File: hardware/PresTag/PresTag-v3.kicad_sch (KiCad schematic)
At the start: 20 parts, among them J201 CONN_02X04, J301 Conn_01x01, J302 Conn_01x01, J303 Conn_01x01, J304 Conn_01x01, J401 CONN_01X02, Q501 Q_NPN_BEC, U1 at25ex321D-UUN, U2 LPS27HHWTR, U302 stm32l412kb, U501 RV-3028-C7

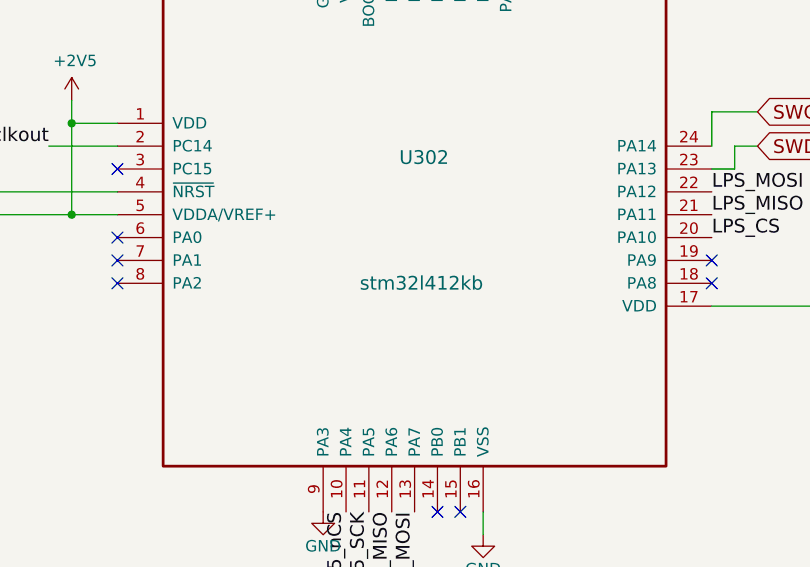
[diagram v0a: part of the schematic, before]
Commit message: revise prestag
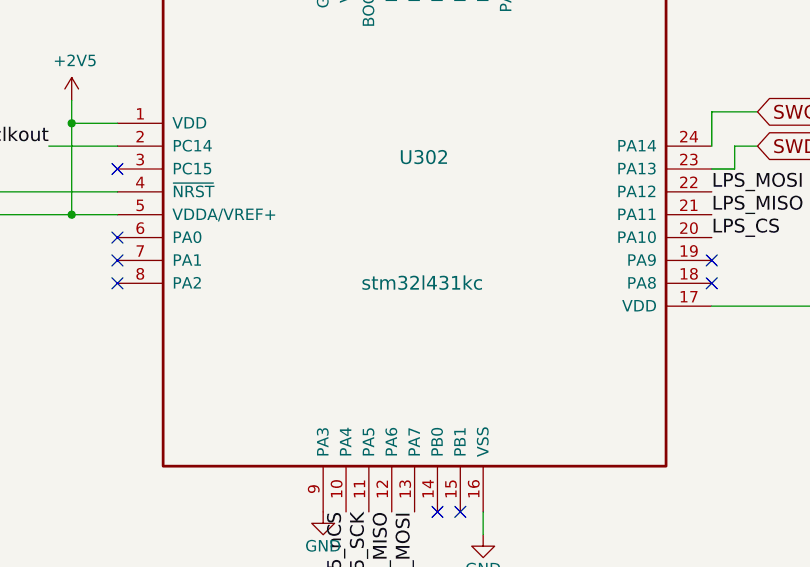
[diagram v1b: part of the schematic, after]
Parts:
- U2: footprint QFN_HHWTR_STM -> lib_fp:LPS27HHWTR
- U302: value stm32l412kb -> stm32l431kc; DISTPN 497-STM32L412K8U6-ND -> 511-STM32L431KCU6; MPN STM32L412K8U6 -> STM32L431KCU6
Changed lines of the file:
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@@
       (effects (font (size 1.524 1.524)) (justify right))
     )
-    (property "Value" "stm32l412kb" (id 1) (at 128.27 93.98 0)
+    (property "Value" "stm32l431kc" (id 1) (at 128.27 93.98 0)
       (effects (font (size 1.524 1.524)) (justify right))
     )
@@
       (effects (font (size 1.524 1.524)) hide)
     )
-    (property "DISTPN" "497-STM32L412K8U6-ND" (id 5) (at 87.63 76.2 0)
-      (effects (font (size 1.524 1.524)) hide)
-    )
-    (property "MPN" "STM32L412K8U6" (id 6) (at 0 152.4 0)
+    (property "DISTPN" "511-STM32L431KCU6" (id 5) (at 87.63 76.2 0)
+      (effects (font (size 1.524 1.524)) hide)
+    )
+    (property "MPN" "STM32L431KCU6" (id 6) (at 0 152.4 0)
       (effects (font (size 1.27 1.27)) hide)
     )
@@
       (effects (font (size 1.524 1.524)))
     )
-    (property "Footprint" "QFN_HHWTR_STM" (id 2) (at 80.645 132.715 0)
+    (property "Footprint" "lib_fp:LPS27HHWTR" (id 2) (at 80.645 132.715 0)
       (effects (font (size 1.524 1.524)) hide)
     )
@@
     )
     (path "/00000000-0000-0000-0000-000060c8320f"
-      (reference "U2") (unit 1) (value "LPS27HHWTR") (footprint "QFN_HHWTR_STM")
+      (reference "U2") (unit 1) (value "LPS27HHWTR") (footprint "lib_fp:LPS27HHWTR")
     )
     (path "/00000000-0000-0000-0000-000058a7531d"
-      (reference "U302") (unit 1) (value "stm32l412kb") (footprint "Package_DFN_QFN:QFN-32-1EP_5x5mm_P0.5mm_EP3.45x3.45mm")
+      (reference "U302") (unit 1) (value "stm32l431kc") (footprint "Package_DFN_QFN:QFN-32-1EP_5x5mm_P0.5mm_EP3.45x3.45mm")
     )
     (path "/00000000-0000-0000-0000-00005ef60ddb"
